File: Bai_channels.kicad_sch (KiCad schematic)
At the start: 24 parts, among them J2 5019514000, U1 ATmega328-P, U2 LM7805_TO220

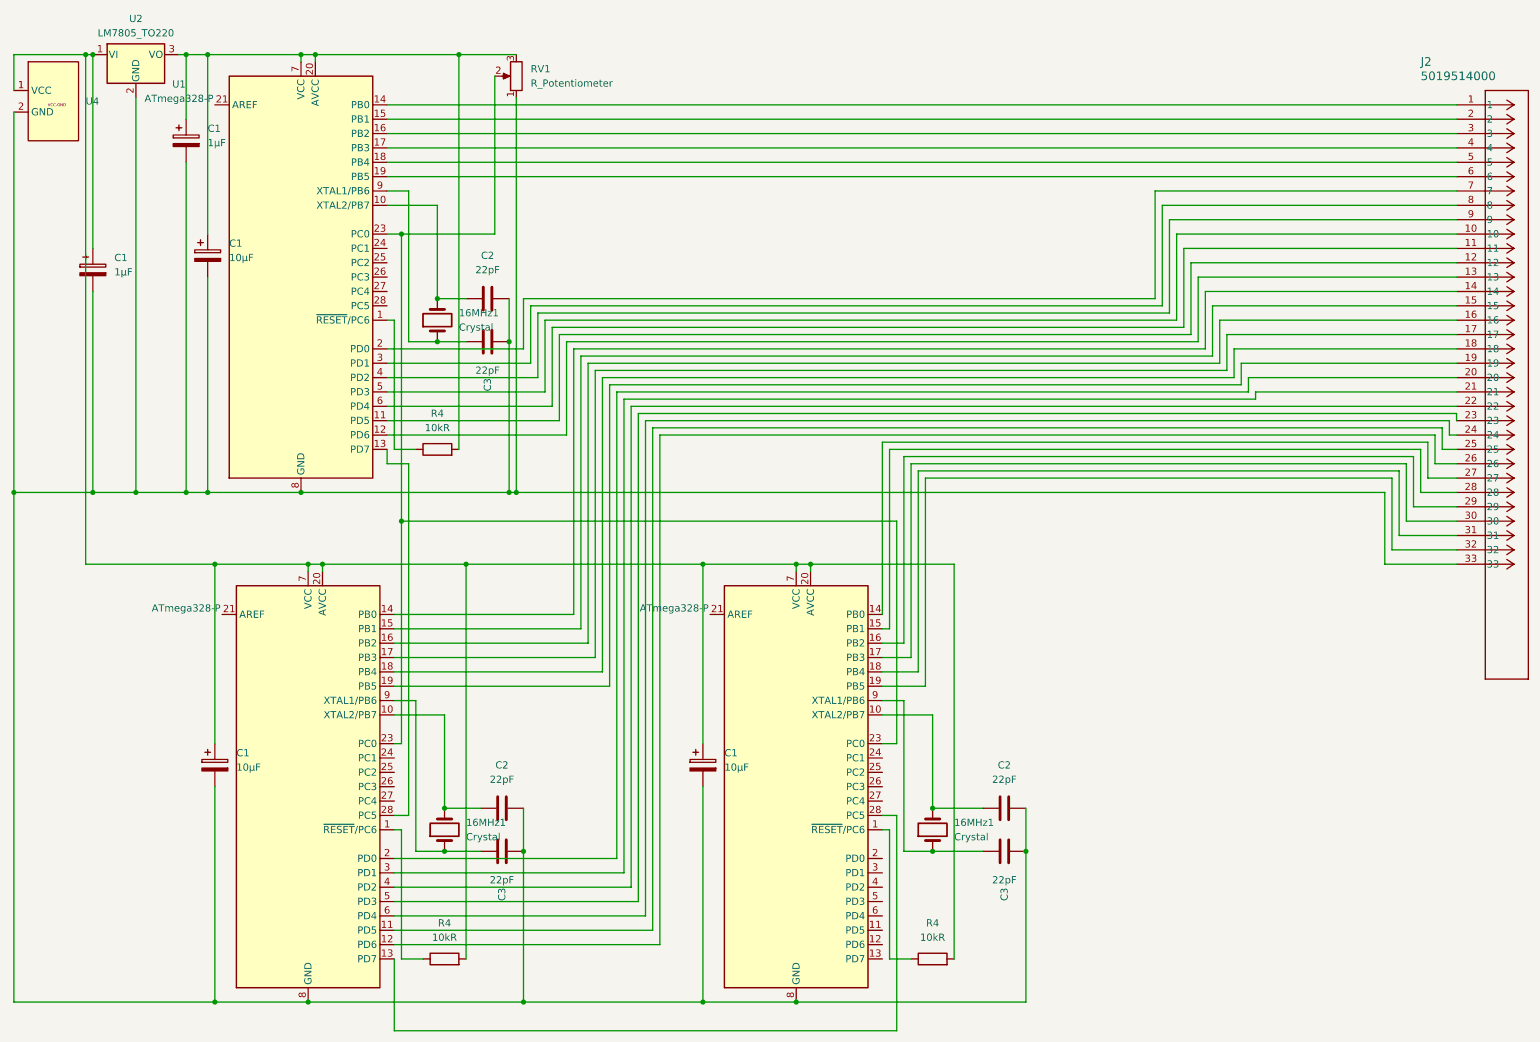
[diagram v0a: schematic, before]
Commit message: 16 channel
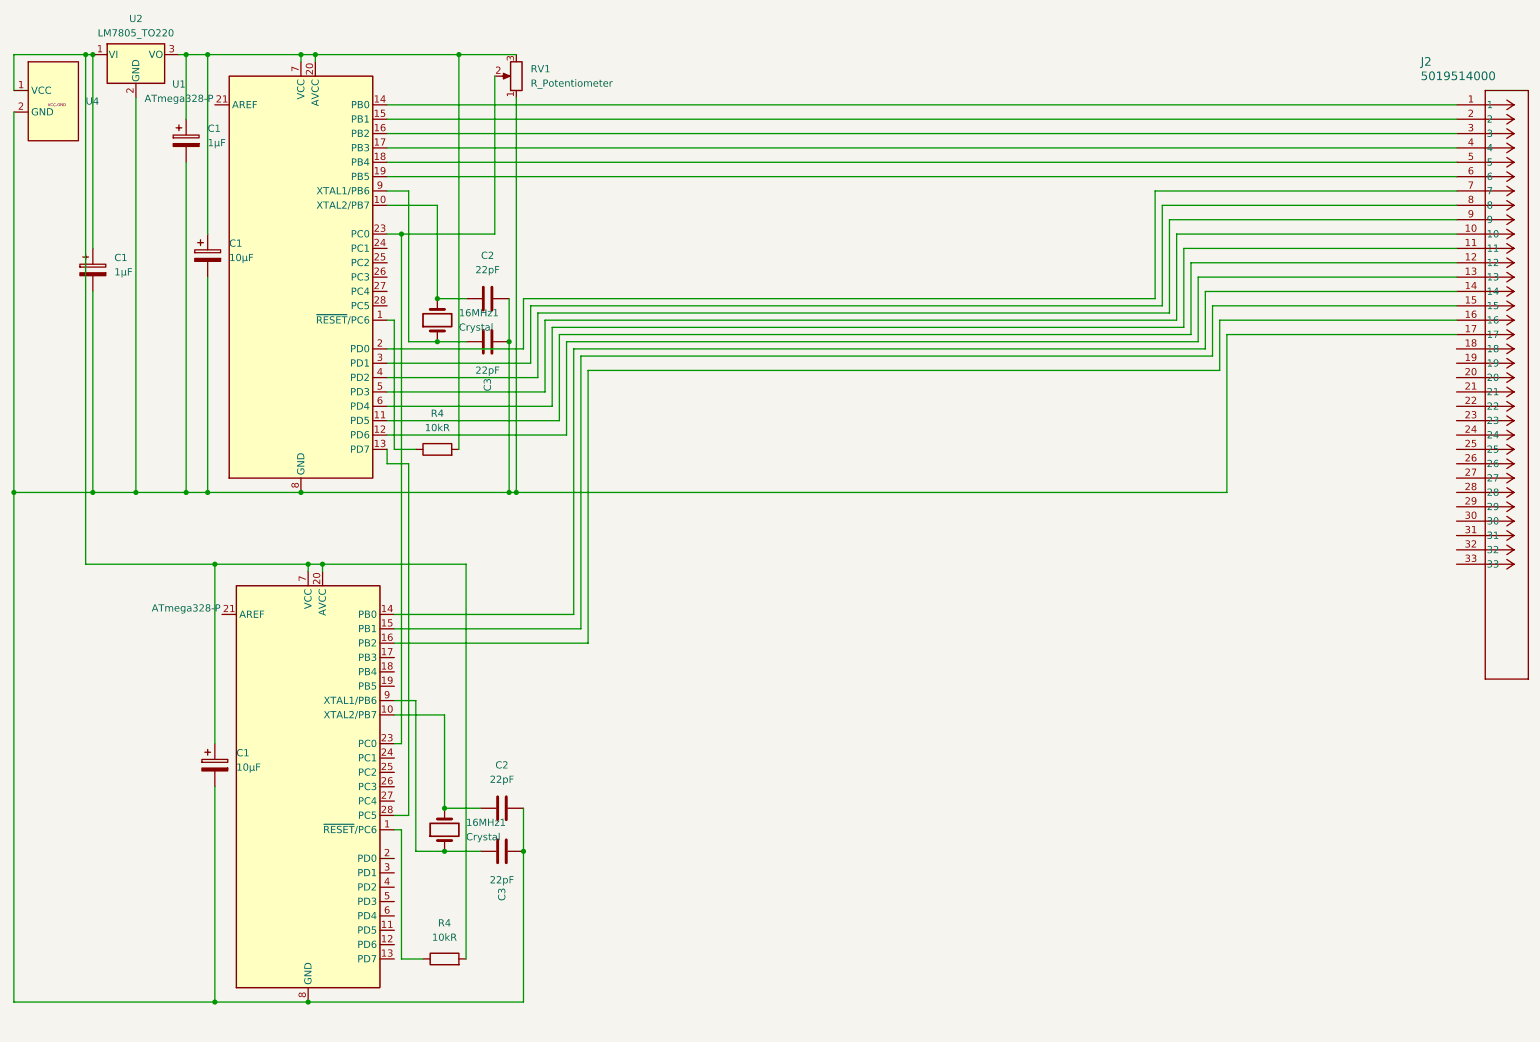
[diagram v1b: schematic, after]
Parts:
- removed 16MHz1: Crystal, Crystal:Crystal_HC49-4H_Vertical, symbol Device:Crystal
- removed C1: 10µF, custom:capacitor, symbol Device:C_Polarized
- removed C2, C3: 22pF, custom:capacitor, symbol Device:C
- removed R4: 10kR, custom:R, symbol Device:R
- removed U1: ATmega328-P, Package_DIP:DIP-28_W7.62mm_Socket, symbol MCU_Microchip_ATmega:ATmega328-P
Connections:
- net at C1.2, C1.2, C1.2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: now also J2.17; no longer J2.33
- net at U1.11 (PD5): no longer J2.25
- net at U1.12 (PD6): no longer J2.26
- net at U1.17 (PB3): no longer J2.17
- net at U1.18 (PB4): no longer J2.18
- net at U1.19 (PB5): no longer J2.19
- net at U1.2 (PD0): no longer J2.20
- net at U1.3 (PD1): no longer J2.21
- net at U1.4 (PD2): no longer J2.22
- net at U1.5 (PD3): no longer J2.23
- net at U1.6 (PD4): no longer J2.24
